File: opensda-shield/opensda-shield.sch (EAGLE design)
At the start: 17 parts, among them IC1 74LVC125, IC2 74LVC125, J1 61302011121, J2 61302011121, J3 61300211121, J4 CORTEX_DEBUG_PTH, J5 61301511121

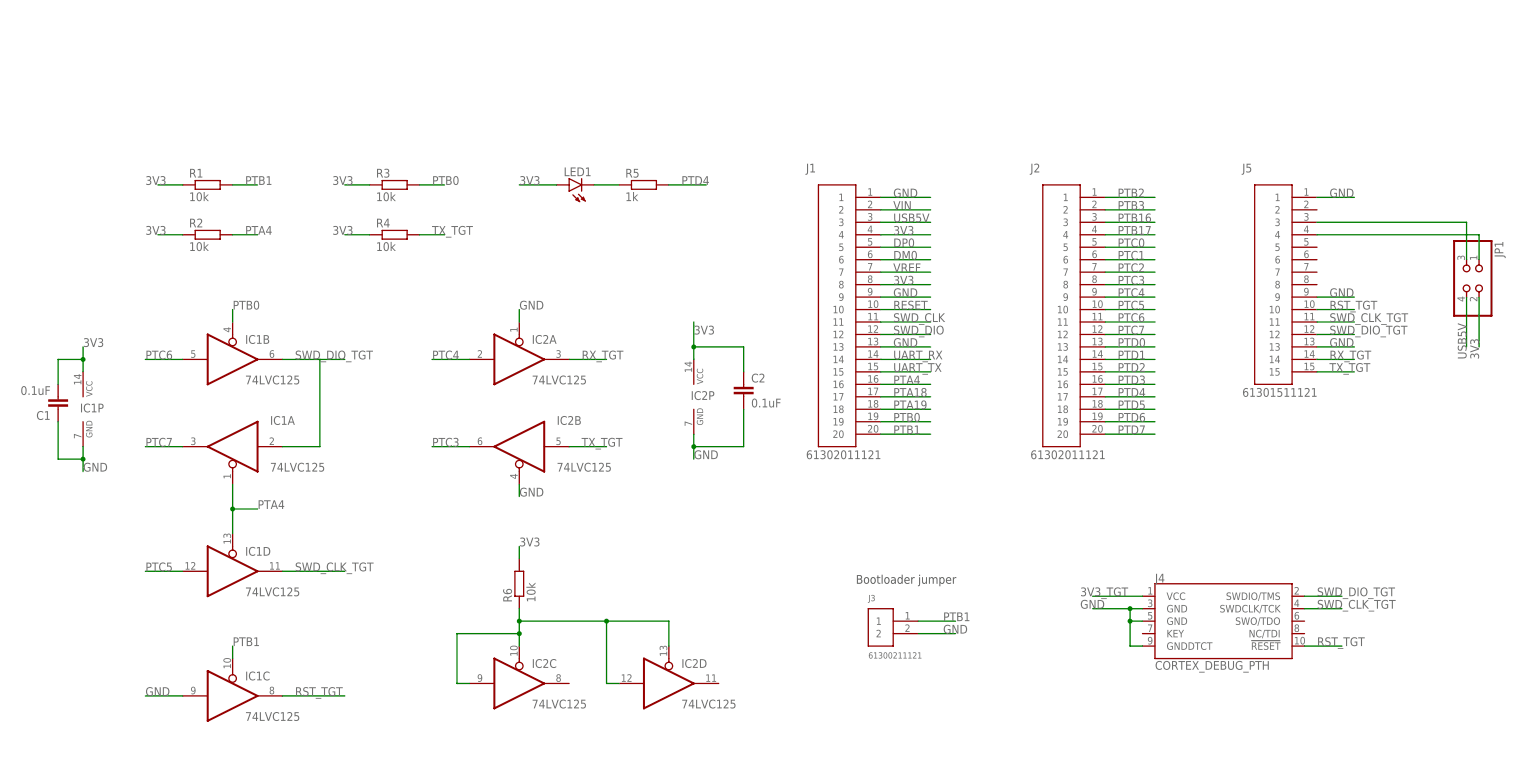
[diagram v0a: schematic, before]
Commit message: Zmeny z e-mailu
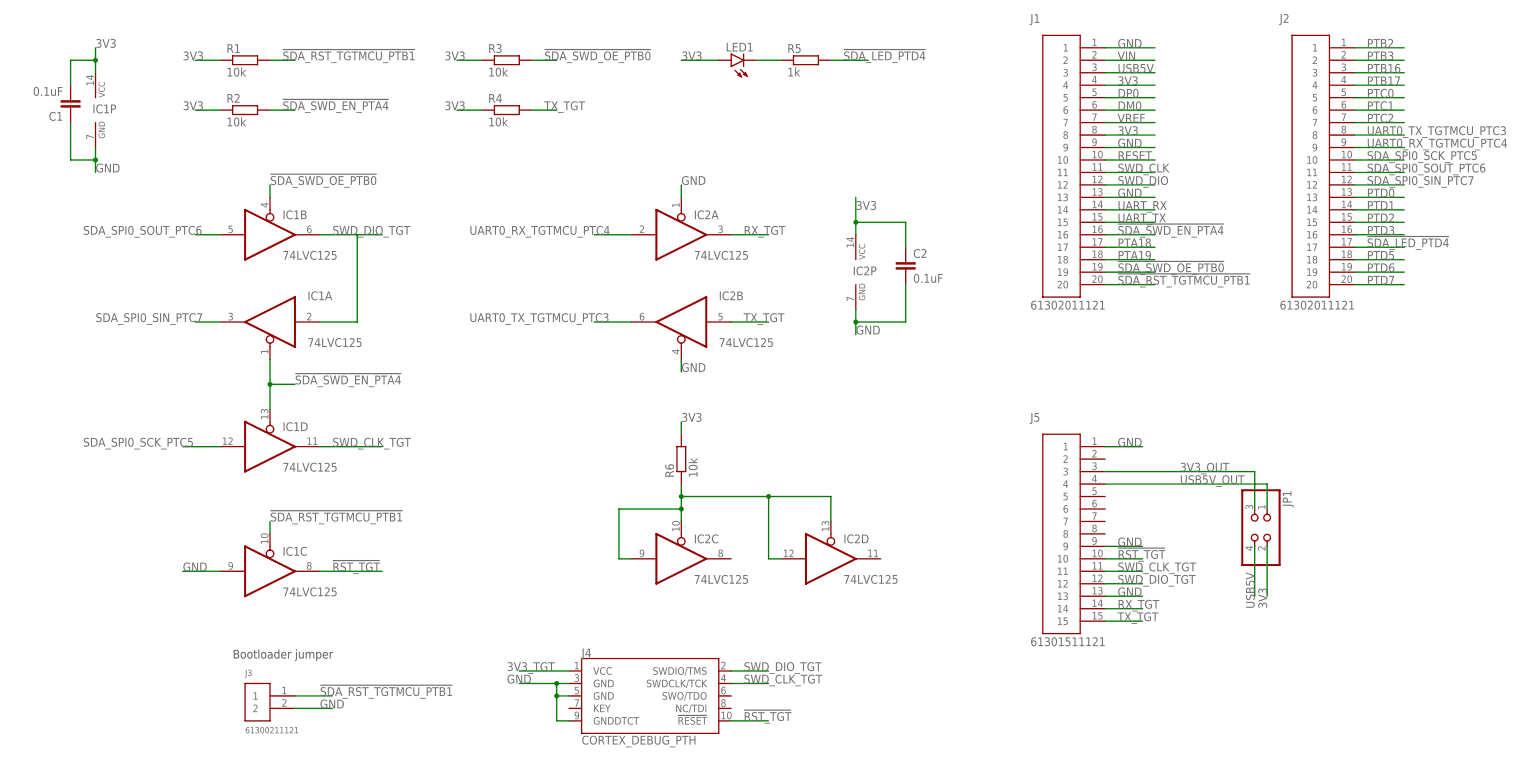
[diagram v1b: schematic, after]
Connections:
- net N$1 renamed 3V3_OUT
- net N$3 renamed USB5V_OUT
- net PTA4 renamed !SDA_SWD_EN_PTA4
- net PTB0 renamed !SDA_SWD_OE_PTB0
- net PTB1 renamed !SDA_RST_TGTMCU_PTB1
- net PTC3 renamed UART0_TX_TGTMCU_PTC3
- net PTC4 renamed UART0_RX_TGTMCU_PTC4
- net PTC5 renamed SDA_SPI0_SCK_PTC5
- net PTC6 renamed SDA_SPI0_SOUT_PTC6
- net PTC7 renamed SDA_SPI0_SIN_PTC7
- net PTD4 renamed !SDA_LED_PTD4
- net RST_TGT renamed !RST_TGT
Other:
- moved on the sheet: C1, C2, IC1A, IC1B, IC1C, IC1D, IC1P, IC2A, IC2B, IC2C, IC2D, IC2P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
